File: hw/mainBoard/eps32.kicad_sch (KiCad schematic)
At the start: 13 parts, among them SW1 SW_Push, SW2 SW_Push, U1 ESP32-WROOM-E, U4 TLV76133DCYR

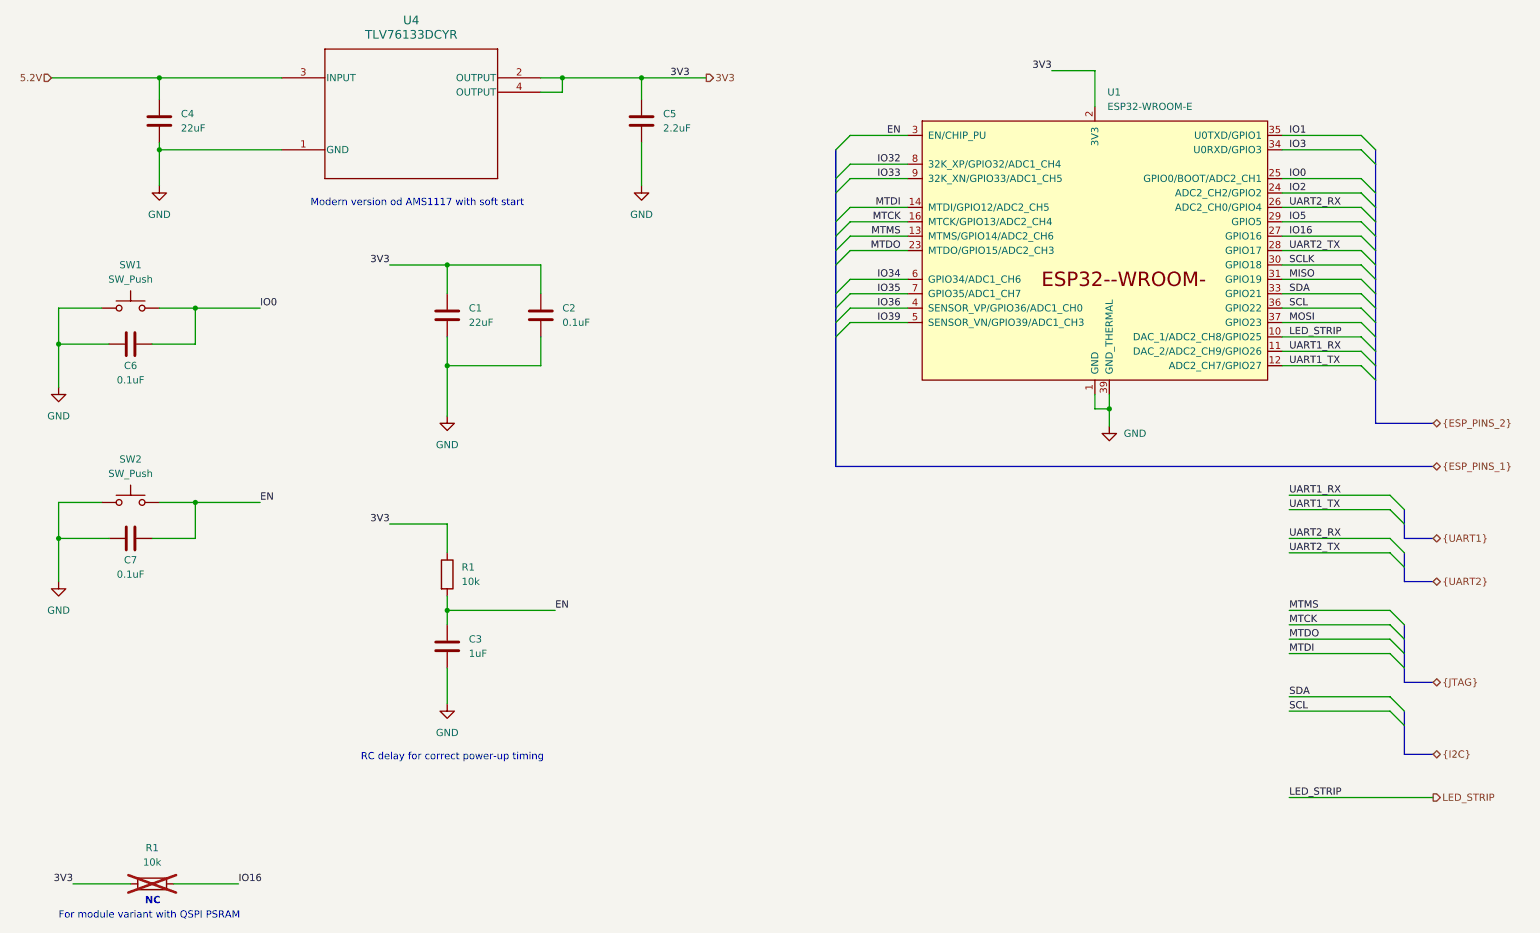
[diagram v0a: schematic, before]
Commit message: schematka
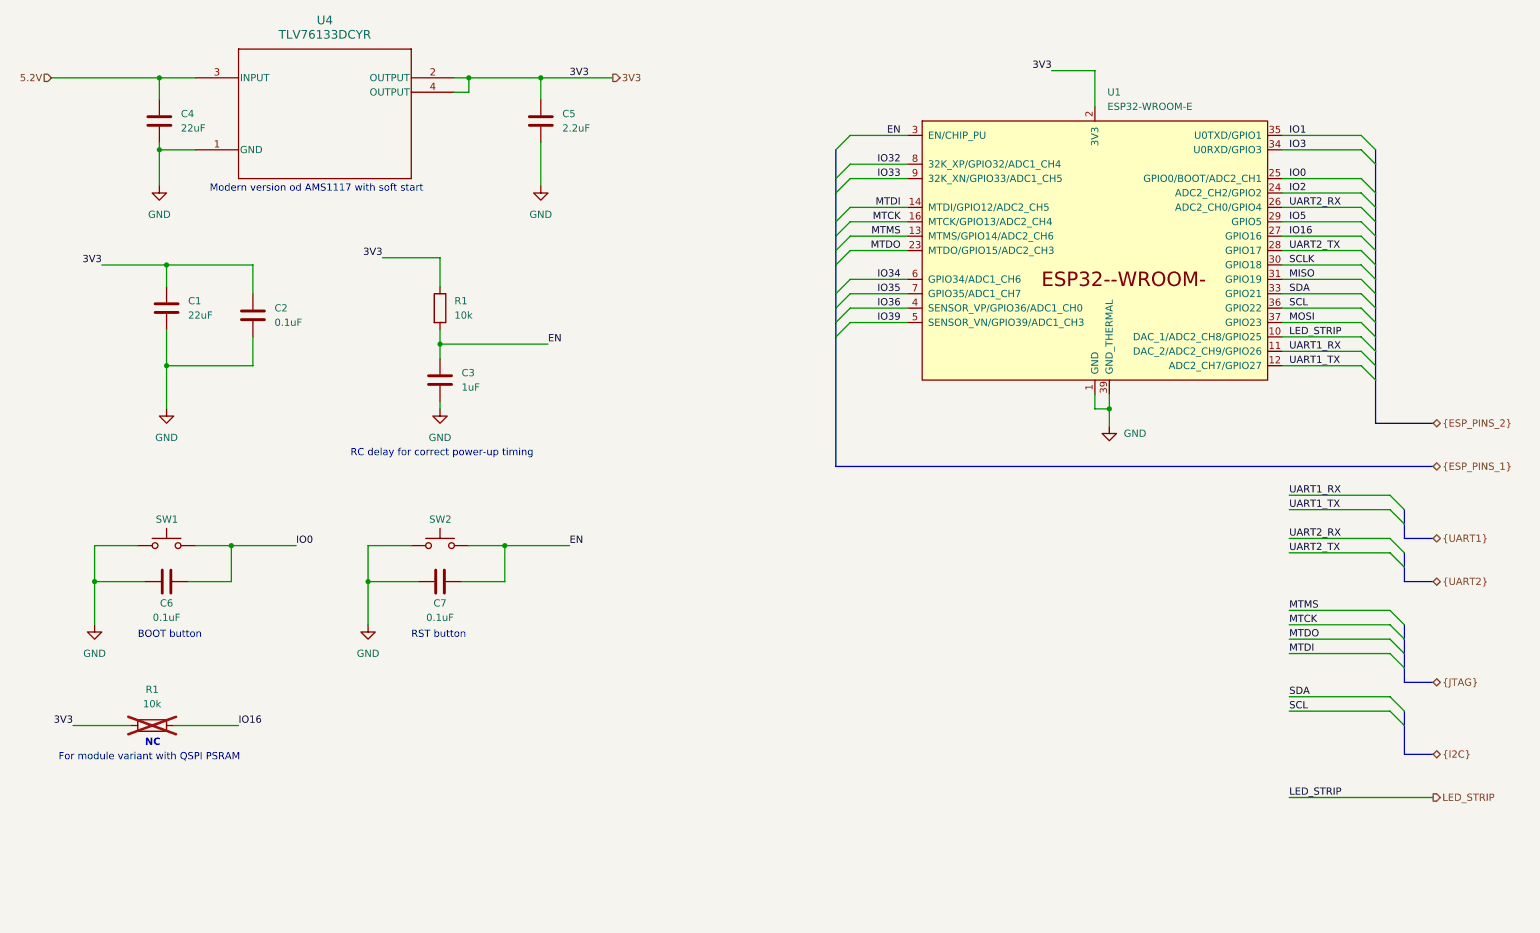
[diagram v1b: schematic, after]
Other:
- note added: "BOOT button"
- note added: "RST button"
- moved on the sheet: C1, C2, C3, C5, C6, C7, R1, SW1, SW2, U4
